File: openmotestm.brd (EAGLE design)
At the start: 24.4 x 34 mm, 49 parts

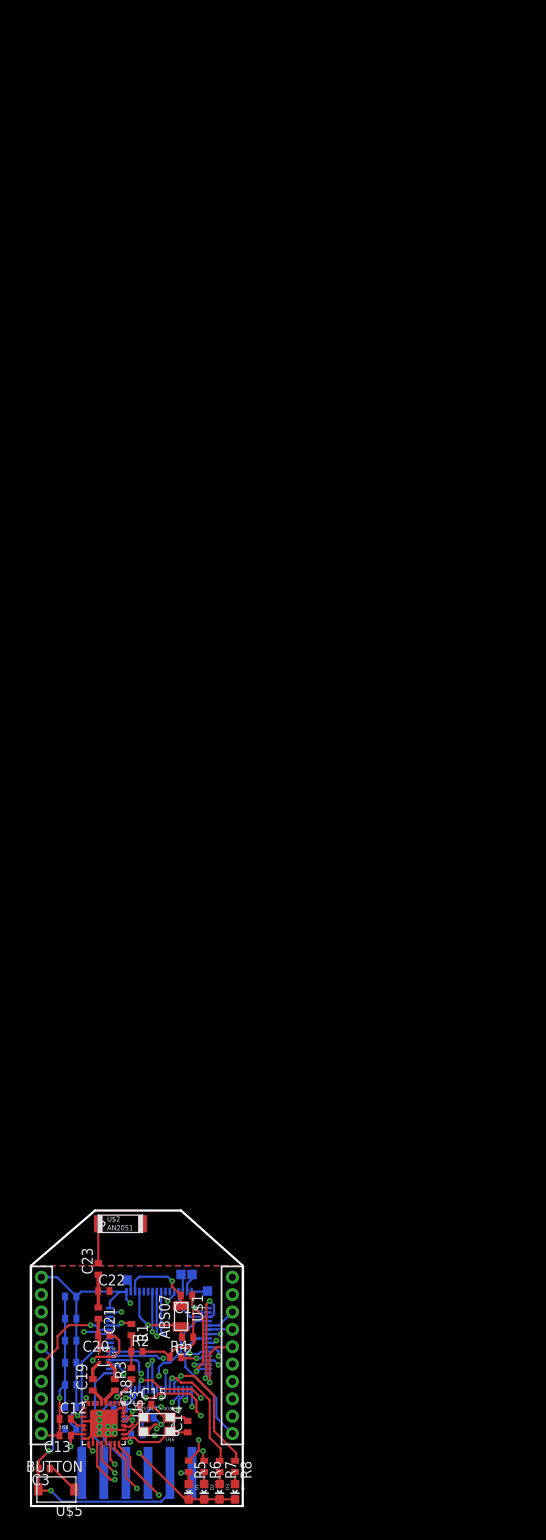
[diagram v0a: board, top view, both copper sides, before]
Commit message: right position in brd.
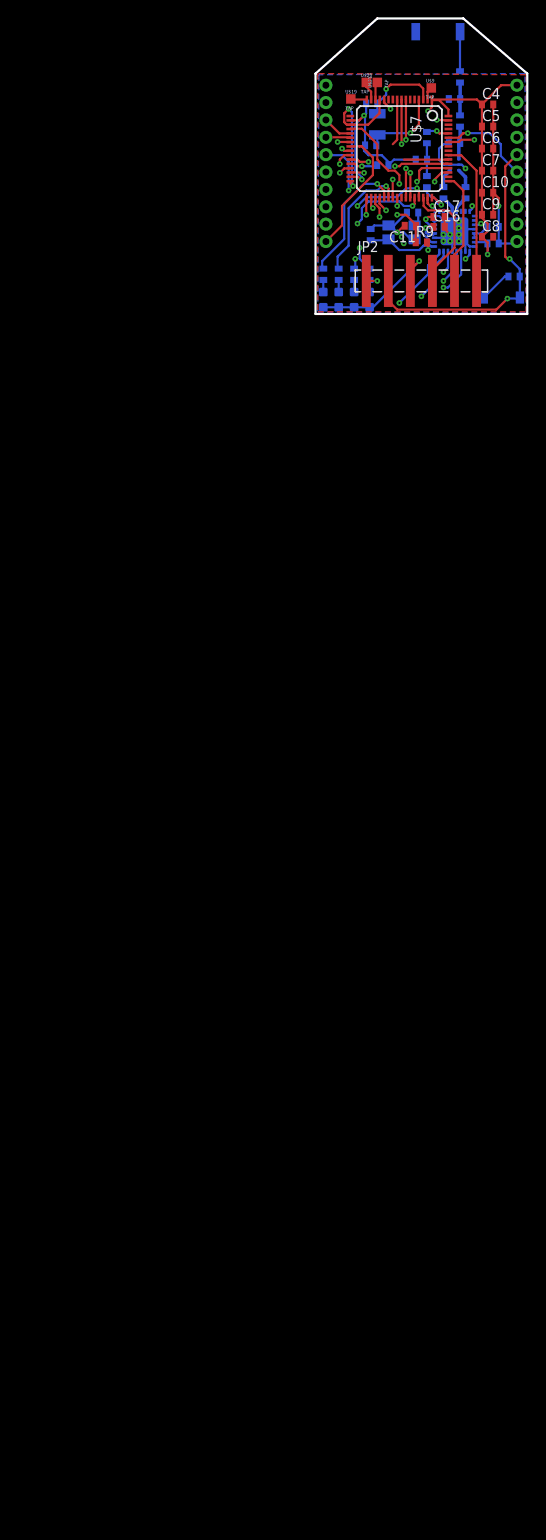
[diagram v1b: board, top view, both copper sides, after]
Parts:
- moved C3 147.6 mm to (56.1, 187.3), flipped to the bottom
- moved U$5 146.6 mm to (54.7, 184.9), flipped to the bottom
- moved C12 145.9 mm to (53.7, 193.0), flipped to the bottom
- moved C13 145.9 mm to (53.7, 191.1), flipped to the bottom
- moved C10 145.4 mm to (53.1, 197.0), flipped to the top
- moved C4 145.4 mm to (53.1, 207.1), flipped to the top
- moved C5 145.4 mm to (53.1, 204.6), flipped to the top
- moved C7 145.4 mm to (53.1, 199.5), flipped to the top
- moved C9 145.4 mm to (53.1, 194.4), flipped to the top
- moved C6 145.4 mm to (53.1, 202.1), flipped to the top
- moved C8 145.4 mm to (53.1, 191.9), flipped to the top
- moved C19 143.8 mm to (50.5, 197.0), flipped to the bottom
- moved C21 143.5 mm to (49.9, 205.2), flipped to the bottom
- moved C23 143.5 mm to (49.9, 210.3), flipped to the bottom
- moved C20 143.1 mm to (49.3, 202.7), flipped to the bottom
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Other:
- outline, holes or cut-outs redrawn
